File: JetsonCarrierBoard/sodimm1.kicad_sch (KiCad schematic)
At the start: 12 parts

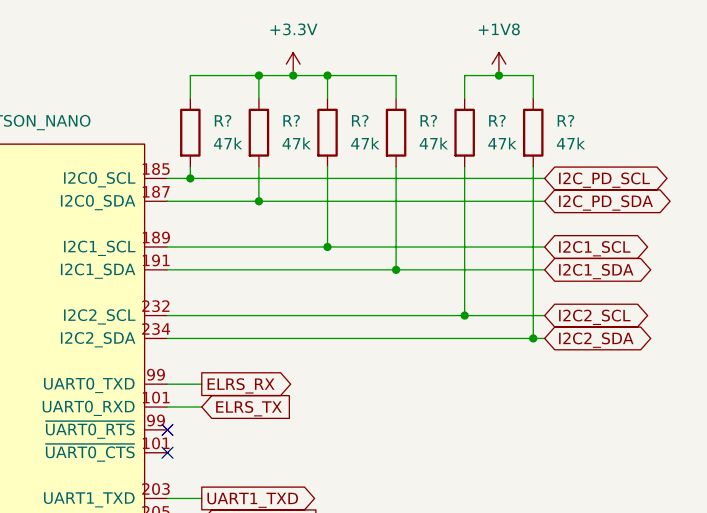
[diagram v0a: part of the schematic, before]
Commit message: GPIO wiring
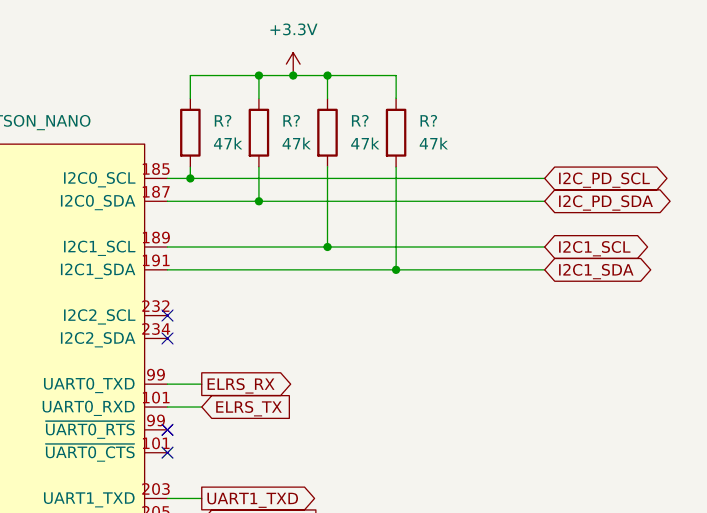
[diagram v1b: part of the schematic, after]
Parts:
- removed R? (x2): 47k, symbol Device:R
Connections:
- net I2C2_SCL: no longer names the net of J?.232 (I2C2_SCL)
- net I2C2_SDA: no longer names the net of J?.234 (I2C2_SDA)
- no-connect marks 7 -> 9
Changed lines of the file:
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@@
   (junction (at 119.38 109.22) (diameter 0) (color 0 0 0 0)
   )
-  (junction (at 204.47 21.59) (diameter 0) (color 0 0 0 0)
-  )
   (junction (at 119.38 43.18) (diameter 0) (color 0 0 0 0)
   )
@@
   )
   (junction (at 119.38 129.54) (diameter 0) (color 0 0 0 0)
-  )
-  (junction (at 200.66 48.26) (diameter 0) (color 0 0 0 0)
-  )
-  (junction (at 208.28 50.8) (diameter 0) (color 0 0 0 0)
   )
   (junction (at 119.38 114.3) (diameter 0) (color 0 0 0 0)
@@
   (no_connect (at 167.64 63.5))
   (no_connect (at 167.64 60.96))
+  (no_connect (at 167.64 50.8))
+  (no_connect (at 167.64 48.26))
   (no_connect (at 167.64 113.03))
   (wire (pts (xy 119.38 124.46) (xy 119.38 127))
@@
     (stroke (width 0) (type default) (color 0 0 0 0))
   )
-  (wire (pts (xy 200.66 24.13) (xy 200.66 21.59))
-    (stroke (width 0) (type default) (color 0 0 0 0))
-  )
   (wire (pts (xy 167.64 55.88) (xy 171.45 55.88))
     (stroke (width 0) (type default) (color 0 0 0 0))
@@
     (stroke (width 0) (type default) (color 0 0 0 0))
   )
-  (wire (pts (xy 208.28 50.8) (xy 208.28 31.75))
-    (stroke (width 0) (type default) (color 0 0 0 0))
-  )
   (wire (pts (xy 119.38 38.1) (xy 119.38 40.64))
     (stroke (width 0) (type default) (color 0 0 0 0))
@@
     (stroke (width 0) (type default) (color 0 0 0 0))
   )
-  (wire (pts (xy 167.64 50.8) (xy 208.28 50.8))
-    (stroke (width 0) (type default) (color 0 0 0 0))
-  )
   (wire (pts (xy 170.18 121.92) (xy 170.18 124.46))
     (stroke (width 0) (type default) (color 0 0 0 0))
@@
     (stroke (width 0) (type default) (color 0 0 0 0))
   )
-  (wire (pts (xy 204.47 21.59) (xy 208.28 21.59))
-    (stroke (width 0) (type default) (color 0 0 0 0))
-  )
   (wire (pts (xy 119.38 147.32) (xy 121.92 147.32))
     (stroke (width 0) (type default) (color 0 0 0 0))
@@
     (stroke (width 0) (type default) (color 0 0 0 0))
   )
-  (wire (pts (xy 167.64 48.26) (xy 200.66 48.26))
-    (stroke (width 0) (type default) (color 0 0 0 0))
-  )
   (wire (pts (xy 119.38 50.8) (xy 119.38 53.34))
     (stroke (width 0) (type default) (color 0 0 0 0))
@@
     (stroke (width 0) (type default) (color 0 0 0 0))
   )
-  (wire (pts (xy 200.66 21.59) (xy 204.47 21.59))
-    (stroke (width 0) (type default) (color 0 0 0 0))
-  )
   (wire (pts (xy 170.18 154.94) (xy 170.18 157.48))
     (stroke (width 0) (type default) (color 0 0 0 0))
@@
     (stroke (width 0) (type default) (color 0 0 0 0))
   )
-  (wire (pts (xy 208.28 21.59) (xy 208.28 24.13))
-    (stroke (width 0) (type default) (color 0 0 0 0))
-  )
   (wire (pts (xy 177.8 35.56) (xy 177.8 31.75))
     (stroke (width 0) (type default) (color 0 0 0 0))
@@
     (stroke (width 0) (type default) (color 0 0 0 0))
   )
-  (wire (pts (xy 200.66 48.26) (xy 200.66 31.75))
-    (stroke (width 0) (type default) (color 0 0 0 0))
-  )
   (wire (pts (xy 119.38 68.58) (xy 119.38 71.12))
     (stroke (width 0) (type default) (color 0 0 0 0))
@@
     (stroke (width 0) (type default) (color 0 0 0 0))
   )
-  (wire (pts (xy 200.66 48.26) (xy 209.55 48.26))
-    (stroke (width 0) (type default) (color 0 0 0 0))
-  )
   (wire (pts (xy 167.64 90.17) (xy 171.45 90.17))
     (stroke (width 0) (type default) (color 0 0 0 0))
@@
     (stroke (width 0) (type default) (color 0 0 0 0))
   )
-  (wire (pts (xy 208.28 50.8) (xy 209.55 50.8))
-    (stroke (width 0) (type default) (color 0 0 0 0))
-  )
   (wire (pts (xy 119.38 134.62) (xy 119.38 137.16))
     (stroke (width 0) (type default) (color 0 0 0 0))
@@
     (effects (font (size 1.27 1.27)) (justify left))
     (property "Intersheet References" "${INTERSHEET_REFS}" (id 0) (at 215.1683 102.7906 0)
-      (effects (font (size 1.27 1.27)) (justify left) hide)
-    )
-  )
-  (global_label "I2C2_SCL" (shape bidirectional) (at 209.55 48.26 0) (fields_autoplaced)
-    (effects (font (size 1.27 1.27)) (justify left))
-    (property "Intersheet References" "${INTERSHEET_REFS}" (id 0) (at 220.7321 48.1806 0)
-      (effects (font (size 1.27 1.27)) (justify left) hide)
-    )
-  )
-  (global_label "I2C2_SDA" (shape bidirectional) (at 209.55 50.8 0) (fields_autoplaced)
-    (effects (font (size 1.27 1.27)) (justify left))
-    (property "Intersheet References" "${INTERSHEET_REFS}" (id 0) (at 220.7926 50.7206 0)
       (effects (font (size 1.27 1.27)) (justify left) hide)
     )
@@
     )
     (pin "1")
-  )
-  (symbol (lib_id "Device:R") (at 208.28 27.94 0) (unit 1)
-    (in_bom yes) (on_board yes) (fields_autoplaced)
-    (property "Reference" "R?" (id 0) (at 210.82 26.6699 0)
-      (effects (font (size 1.27 1.27)) (justify left))
-    )
-    (property "Value" "47k" (id 1) (at 210.82 29.2099 0)
-      (effects (font (size 1.27 1.27)) (justify left))
-    )
-    (property "Footprint" "" (id 2) (at 206.502 27.94 90)
-      (effects (font (size 1.27 1.27)) hide)
-    )
-    (property "Datasheet" "~" (id 3) (at 208.28 27.94 0)
-      (effects (font (size 1.27 1.27)) hide)
-    )
-    (pin "1")
-    (pin "2")
   )
   (symbol (lib_id "Device:D_TVS") (at 191.77 120.65 90) (unit 1)
@@
     (pin "2")
   )
-  (symbol (lib_id "Device:R") (at 200.66 27.94 0) (unit 1)
-    (in_bom yes) (on_board yes) (fields_autoplaced)
-    (property "Reference" "R?" (id 0) (at 203.2 26.6699 0)
-      (effects (font (size 1.27 1.27)) (justify left))
-    )
-    (property "Value" "47k" (id 1) (at 203.2 29.2099 0)
-      (effects (font (size 1.27 1.27)) (justify left))
-    )
-    (property "Footprint" "" (id 2) (at 198.882 27.94 90)
-      (effects (font (size 1.27 1.27)) hide)
-    )
-    (property "Datasheet" "~" (id 3) (at 200.66 27.94 0)
-      (effects (font (size 1.27 1.27)) hide)
-    )
-    (pin "1")
-    (pin "2")
-  )
   (symbol (lib_id "Device:R") (at 177.8 27.94 0) (unit 1)
     (in_bom yes) (on_board yes) (fields_autoplaced)
@@
       (effects (font (size 1.27 1.27)) hide)
     )
-    (pin "1")
-  )
-  (symbol (lib_id "power:+1V8") (at 204.47 21.59 0) (unit 1)
-    (in_bom yes) (on_board yes) (fields_autoplaced)
-    (property "Reference" "#PWR?" (id 0) (at 204.47 25.4 0)
-      (effects (font (size 1.27 1.27)) hide)
-    )
-    (property "Value" "+1V8" (id 1) (at 204.47 16.51 0))
-    (property "Footprint" "" (id 2) (at 204.47 21.59 0)
-      (effects (font (size 1.27 1.27)) hide)
-    )
-    (property "Datasheet" "" (id 3) (at 204.47 21.59 0)
-      (effects (font (size 1.27 1.27)) hide)
-    )
